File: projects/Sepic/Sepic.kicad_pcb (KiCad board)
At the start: 2 copper layers, 48.3 x 25.4 mm, 31 parts, among them P1 V_in+, P10 V_out+, P11 V_out-, P12 NC, P13 NC, P14 NC, P15 NC, P16 NC, P2 GND, P3 JST_In, P4 En, P5 V_in+, P6 V_in-, P7 NC, P8 V_out+, P9 GND, U1 LT1370

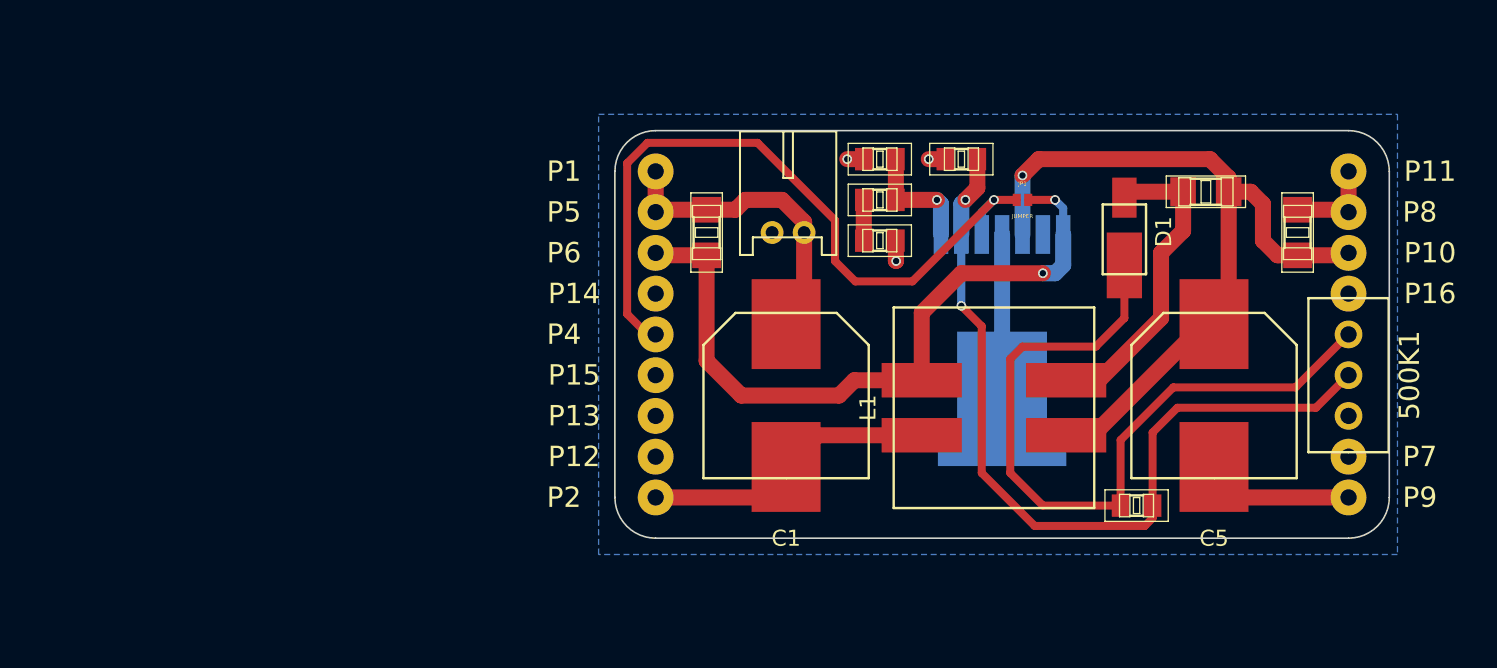
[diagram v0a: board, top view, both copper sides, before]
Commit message: working on sepic
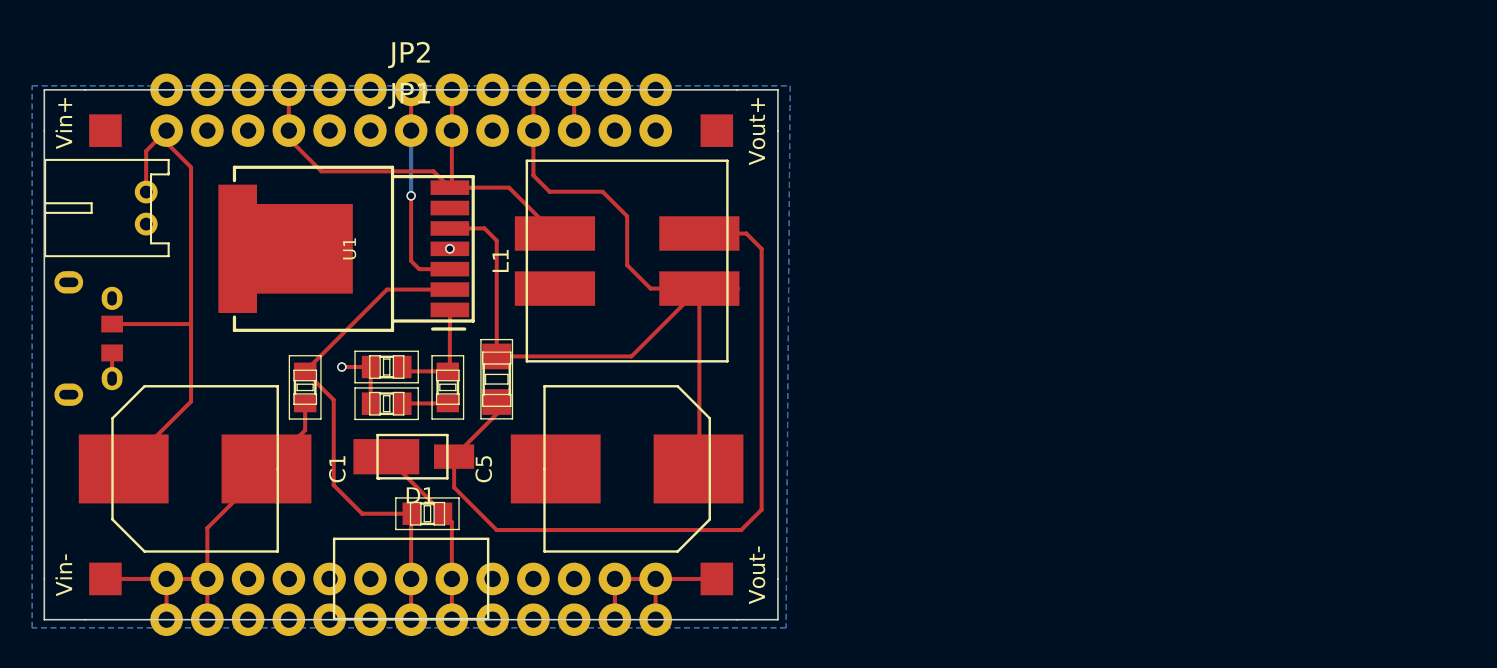
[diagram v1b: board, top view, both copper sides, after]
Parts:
- removed R4, R5: 0R, frep:R1206
- added 500K2: POT, frep:Trimmer, F.Cu at (114.3, 119.4)
- added CON1: USB-MICRO-LOAD, frep:USB_Micro_Load, F.Cu at (93.0, 101.9)
- added JP2: JUMPER3, frep:Pin_Proto_Straight_1x03, F.Cu at (114.3, 86.4)
- added P17: GND, frep:Pin_Proto_Straight_1x01, F.Cu at (127.0, 116.8)
- added P18: V_in+, frep:Pin_Proto_Straight_1x01, F.Cu at (104.1, 86.4)
- added P19: V_in-, frep:Pin_Proto_Straight_1x01, F.Cu at (106.7, 86.4)
- added P20: V_out+, frep:Pin_Proto_Straight_1x01, F.Cu at (121.9, 86.4)
- added P21: V_out-, frep:Pin_Proto_Straight_1x01, F.Cu at (127.0, 86.4)
- added P22: V_out+, frep:Pin_Proto_Straight_1x01, F.Cu at (129.5, 86.4)
- added P23: V_out+, frep:Pin_Proto_Straight_1x01, F.Cu at (124.5, 86.4)
- added P24: GND, frep:Pin_Proto_Straight_1x01, F.Cu at (129.5, 119.4)
- added P25: GND, frep:Pin_Proto_Straight_1x01, F.Cu at (127.0, 119.4)
- added P26: V_out+, frep:Pin_Proto_Straight_1x01, F.Cu at (129.5, 88.9)
- added P27: V_out+, frep:Pin_Proto_Straight_1x01, F.Cu at (127.0, 88.9)
- added P28: GND, frep:Pin_Proto_Straight_1x01, F.Cu at (99.1, 119.4)
- added P29: GND, frep:Pin_Proto_Straight_1x01, F.Cu at (129.5, 116.8)
- added P30: CONN_3X2, frep:Pin_Proto_Straight_2x03, F.Cu at (106.7, 118.1)
- added P31: CONN_3X2, frep:Pin_Proto_Straight_2x03, F.Cu at (121.9, 118.1)
- added P32: CONN_2, frep:Pin_Proto_Straight_1x02, F.Cu at (119.4, 87.6)
- added P33: CONN_2, frep:Pin_Proto_Straight_1x02, F.Cu at (109.2, 87.6)
- JP1: value JUMPER -> JUMPER3; footprint bytelabs:S_JUMPER_2 -> frep:Pin_Proto_Straight_1x03
- P1, P8, P9: footprint frep:Pin_Proto_Straight_1x01 -> frep:SMD_SOLDERPOINT
- P12, P13: value NC -> GND
- P14: value NC -> GND; footprint frep:Pin_Proto_Straight_1x01 -> frep:SMD_SOLDERPOINT
- P15, P16, P7: value NC -> V_in+
- P4: value En -> V_in+
- U1: moved to F.Cu
- moved P7 74.0 mm to (101.6, 88.9)
- moved P16 72.2 mm to (101.6, 86.4)
- moved 500K1 59.8 mm to (114.3, 116.8), turned to 180 degrees
- moved P10 51.4 mm to (121.9, 88.9)
- moved P11 48.3 mm to (124.5, 88.9)
- moved D1 46.1 mm to (114.8, 109.2), turned to 0 degrees
- moved C4 45.7 mm to (119.6, 104.4), turned to 90 degrees
- moved R2 44.2 mm to (115.3, 112.8), turned to 180 degrees
- moved R3 43.3 mm to (107.7, 104.9), turned to 270 degrees
- moved U1 41.0 mm to (110.5, 96.3), turned to 90 degrees
- moved P3 40.0 mm to (97.8, 93.7), turned to 90 degrees
- moved P8 39.7 mm to (133.3, 88.9)
- moved P9 39.7 mm to (133.3, 116.8)
- moved P14 38.6 mm to (95.2, 116.8)
- moved JP1 38.3 mm to (114.3, 88.9)
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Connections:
- L1 pad 3: Net-(JP1-Pad2) -> Net-(JP1-Pad3)
- P12 pad 1: Net-(P12-Pad1) -> GND
- P13 pad 1: Net-(P13-Pad1) -> GND
- P14 pad 1: Net-(P14-Pad1) -> GND
- P15 pad 1: Net-(P15-Pad1) -> Net-(C1-Pad1)
- P16 pad 1: Net-(P16-Pad1) -> Net-(C1-Pad1)
- P4 pad 1: Net-(JP1-Pad1) -> Net-(C1-Pad1)
- P6 pad 1: Net-(JP1-Pad2) -> Net-(JP1-Pad3)
- P7 pad 1: Net-(P7-Pad1) -> Net-(C1-Pad1)
- U1 pad 3: Net-(JP1-Pad1) -> Net-(JP1-Pad2)
- U1 pad 7: Net-(JP1-Pad2) -> Net-(JP1-Pad3)
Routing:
- net Net-(JP1-Pad1): track 46.2 -> 0.00 mm, vias 1 -> 0
- net Net-(500K1-Pad1): track 47.3 -> 12.2 mm
- net Net-(JP1-Pad2): track 44.7 -> 13.3 mm, vias 2 -> 1
- net Net-(C4-Pad1): track 19.8 -> 48.6 mm
- net Net-(JP1-Pad3): track 0.00 -> 28.2 mm
- net Net-(500K1-Pad2): track 51.7 -> 31.2 mm, vias 2 -> 0
- net Net-(C1-Pad1): track 19.5 -> 32.9 mm
- net Net-(C4-Pad2): track 51.9 -> 61.2 mm, vias 1 -> 0
- net Net-(P11-Pad1): track 5.78 -> 2.54 mm
- net GND: track 44.6 -> 42.0 mm, vias 3 -> 2
- net Net-(C3-Pad1): track 7.36 -> 6.81 mm, vias 1 -> 0
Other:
- board size 48.3 x 25.4 mm -> 45.7 x 33 mm
- net class Default: trace_width 1 -> 0.25
- net class signal removed
- board text added: "Vin+"
- board text added: "Vin-"
- board text added: "Vout+"
- board text added: "Vout-"
